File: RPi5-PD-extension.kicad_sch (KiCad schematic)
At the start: 4 parts, among them J1 HDMI0_Plug, J2 HDMI0_Receptacle, J3 HDMI1_Plug, J4 HDMI1_Receptacle

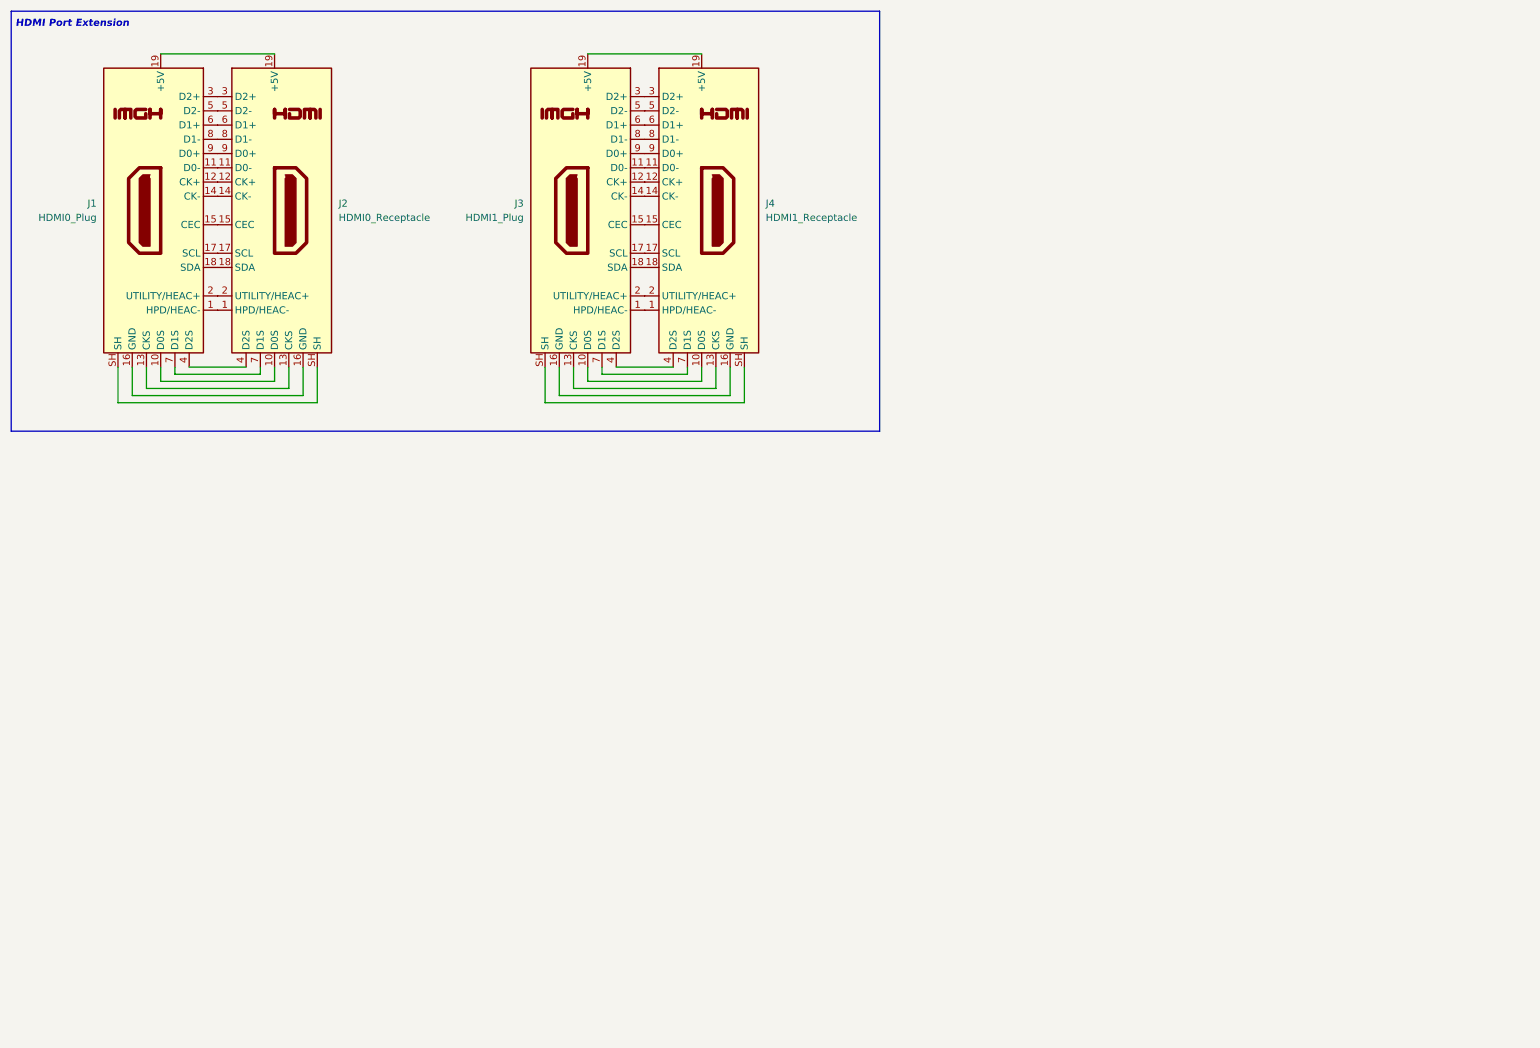
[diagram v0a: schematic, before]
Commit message: Design v1
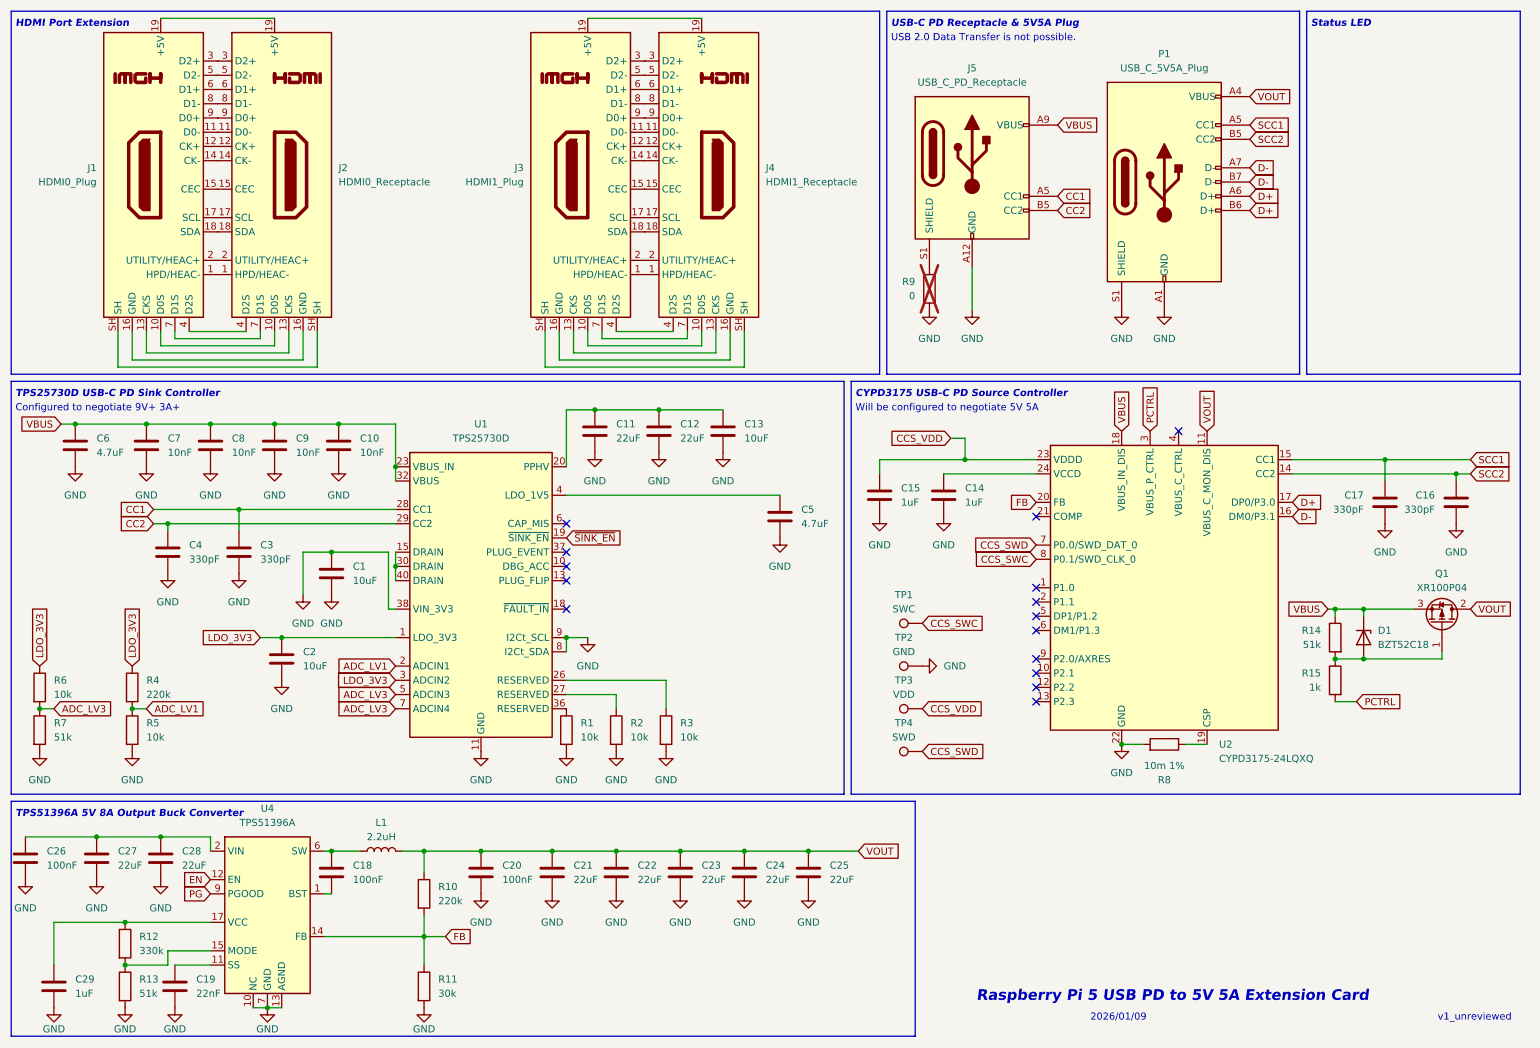
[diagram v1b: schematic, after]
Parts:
- added C1, C13, C2: 10uF, symbol Device:C
- added C10, C7, C8, C9: 10nF, symbol Device:C
- added C11, C12, C21, C22, C23, C24, C25, C27, C28: 22uF, symbol Device:C
- added C14, C15, C29: 1uF, symbol Device:C
- added C16, C17, C3, C4: 330pF, symbol Device:C
- added C18, C20, C26: 100nF, symbol Device:C
- added C19: 22nF, symbol Device:C
- added C5, C6: 4.7uF, symbol Device:C
- added D1: BZT52C18, Diode_SMD:D_SOD-123F, symbol Diode:BZT52Bxx
- added J5: USB_C_PD_Receptacle, symbol Connector:USB_C_Receptacle_PowerOnly_6P
- added L1: 2.2uH, symbol Device:L
- added P1: USB_C_5V5A_Plug, symbol Connector:USB_C_Receptacle_USB2.0_14P
- added Q1: XR100P04, Package_TO_SOT_SMD:TO-252-2, symbol Transistor_FET:SUD50P04-08
- added R1, R2, R3, R5, R6: 10k, symbol Device:R
- added R10, R4: 220k, symbol Device:R
- added R11: 30k, symbol Device:R
- added R12: 330k, symbol Device:R
- added R13, R14, R7: 51k, symbol Device:R
- added R15: 1k, symbol Device:R
- added R8: 10m 1%, symbol Device:R
- added R9: 0, symbol Device:R
- added TP1: SWC, symbol Connector:TestPoint
- added TP2: GND, symbol Connector:TestPoint
- added TP3: VDD, symbol Connector:TestPoint
- added TP4: SWD, symbol Connector:TestPoint
- added U1: TPS25730D, Package_DFN_QFN:Texas_REF0038A_WQFN-38-2EP_6x4mm_P0.4, symbol Interface_USB:TPS25730D
- added U2: CYPD3175-24LQXQ, Package_DFN_QFN:QFN-24-1EP_4x4mm_P0.5mm_EP2.75x2.75mm, symbol Interface_USB:CYPD3175-24LQXQ
- added U4: TPS51396A, Package_DFN_QFN:Texas_RJE0020A_VQFN-20-1EP_3x3mm_P0.45mm_EP0.675x0.76mm, symbol Regulator_Switching:TPS51396A
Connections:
- new net: D1.2 (A), Q1.1 (G), R14.2, R15.1
- new net: C29.1, R12.1, U4.17 (VCC)
- new net: R12.2, R13.1, U4.15 (MODE)
- new net: R3.1, U1.26 (RESERVED)
- new net: C18.2, U4.1 (BST)
- new net: C19.1, U4.11 (SS)
- new net: C18.1, L1.1, U4.19 (SW), U4.20 (SW), U4.6 (SW)
- new net: C26.1, C27.1, C28.1, U4.2 (VIN), U4.3 (VIN), U4.4 (VIN), U4.5 (VIN)
- new net: C11.1, C12.1, C13.1, U1.20 (PPHV)
- new net: U1.15 (DRAIN), U1.30 (DRAIN), U1.40 (DRAIN)
- new net: R2.1, U1.27 (RESERVED)
- new net: R1.1, U1.36 (RESERVED)
- new net: C5.1, U1.4 (LDO_1V5)
- new net: R8.1, U2.19 (CSP)
- new net: C14.1, U2.24 (VCCD)
- new net: J5.S1 (SHIELD), R9.1
- new net ADC_LV1: R4.2, R5.1, U1.2 (ADCIN1)
- new net ADC_LV3: R6.2, R7.1, U1.5 (ADCIN3), U1.7 (ADCIN4)
- new net CC1: C3.1, J5.A5 (CC1), U1.28 (CC1)
- new net CC2: C4.1, J5.B5 (CC2), U1.29 (CC2)
- new net CCS_SWC: TP1.1, U2.8 (P0.1/SWD_CLK_0)
- new net CCS_SWD: TP4.1, U2.7 (P0.0/SWD_DAT_0)
- new net CCS_VDD: C15.1, TP3.1, U2.23 (VDDD)
- new net D+: P1.A6 (D+), P1.B6 (D+), U2.17 (DP0/P3.0)
- new net D-: P1.A7 (D-), P1.B7 (D-), U2.16 (DM0/P3.1)
- new net EN: U4.12 (EN)
- new net FB: R10.2, R11.1, U2.20 (FB), U4.14 (FB)
- new net GND: C1.1, C1.2, C10.2, C11.2, C12.2, C13.2, C14.2, C15.2, C16.2, C17.2, C19.2, C2.2, C20.2, C21.2, C22.2, C23.2, C24.2, C25.2, C26.2, C27.2, C28.2, C29.2, C3.2, C4.2, C5.2, C6.2, C7.2, C8.2, C9.2, J5.A12 (GND), J5.B12 (GND), P1.A1 (GND), P1.A12 (GND), P1.B1 (GND), P1.B12 (GND), P1.S1 (SHIELD), R1.2, R11.2, R13.2, R2.2, R3.2, R5.2, R7.2, R8.2, R9.2, TP2.1, U1.11 (GND), U1.12 (GND), U1.14 (GND), U1.16 (GND), U1.17 (GND), U1.31 (GND), U1.34 (GND), U1.38 (VIN_3V3), U1.39 (GND), U1.8 (I2Ct_SDA), U1.9 (I2Ct_SCL), U2.22 (GND), U2.25 (GND), U4.10 (NC), U4.13 (AGND), U4.16 (NC), U4.18 (GND), U4.21 (GND), U4.7 (GND), U4.8 (GND)
- new net LDO_3V3: C2.1, R4.1, R6.1, U1.1 (LDO_3V3), U1.3 (ADCIN2)
- new net PCTRL: R15.2, U2.3 (VBUS_P_CTRL)
- new net PG: U4.9 (PGOOD)
- new net SCC1: C17.1, P1.A5 (CC1), U2.15 (CC1)
- new net SCC2: C16.1, P1.B5 (CC2), U2.14 (CC2)
- new net VBUS: C10.1, C6.1, C7.1, C8.1, C9.1, D1.1 (K), J5.A9 (VBUS), J5.B9 (VBUS), Q1.3 (S), R14.1, U1.23 (VBUS_IN), U1.32 (VBUS), U2.18 (VBUS_IN_DIS)
- new net VOUT: C20.1, C21.1, C22.1, C23.1, C24.1, C25.1, L1.2, P1.A4 (VBUS), P1.A9 (VBUS), P1.B4 (VBUS), P1.B9 (VBUS), Q1.2 (D), R10.1, U2.11 (VBUS_C_MON_DIS)
- new net ~{SINK_EN}: U1.19 (~{SINK_EN})
- no-connect marks 0 -> 15
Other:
- note added: "2026/01/09"
- note added: "CYPD3175 USB-C PD Source Controller"
- note added: "Configured to negotiate 9V+ 3A+"
- note added: "Raspberry Pi 5 USB PD to 5V 5A Extension Card"
- note added: "Status LED"
- note added: "TPS25730D USB-C PD Sink Controller"
- note added: "TPS51396A 5V 8A Output Buck Converter"
- note added: "USB 2.0 Data Transfer is not possible."
- note added: "USB-C PD Receptacle & 5V5A Plug"
- note added: "Will be configured to negotiate 5V 5A"
- note added: "v1_unreviewed"
- moved on the sheet: J1, J2, J3, J4
